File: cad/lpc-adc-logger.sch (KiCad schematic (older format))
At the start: 26 parts, among them J1 SD_CARD, J2 UART, J3 I2C, J4 ANALOG IN, J5 SWD, J6 GPIO, SW2 RESET, SW3 FLUSH, U1 LPC1114FN28

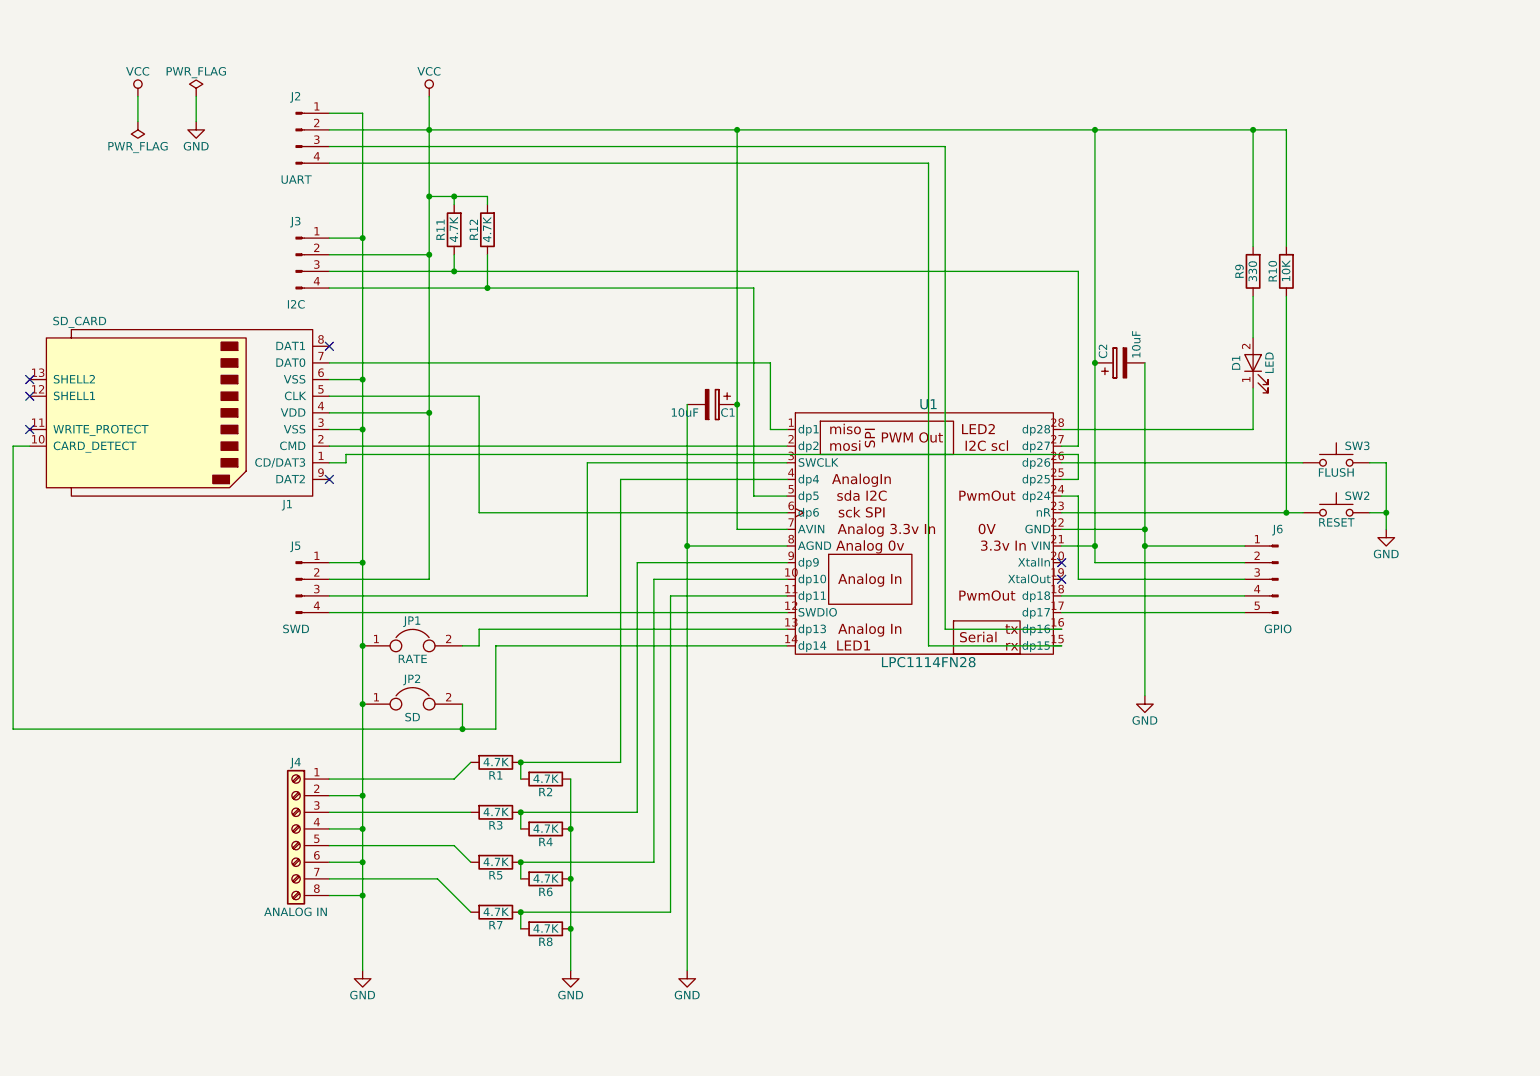
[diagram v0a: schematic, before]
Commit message: [WIP] Added SPI header.
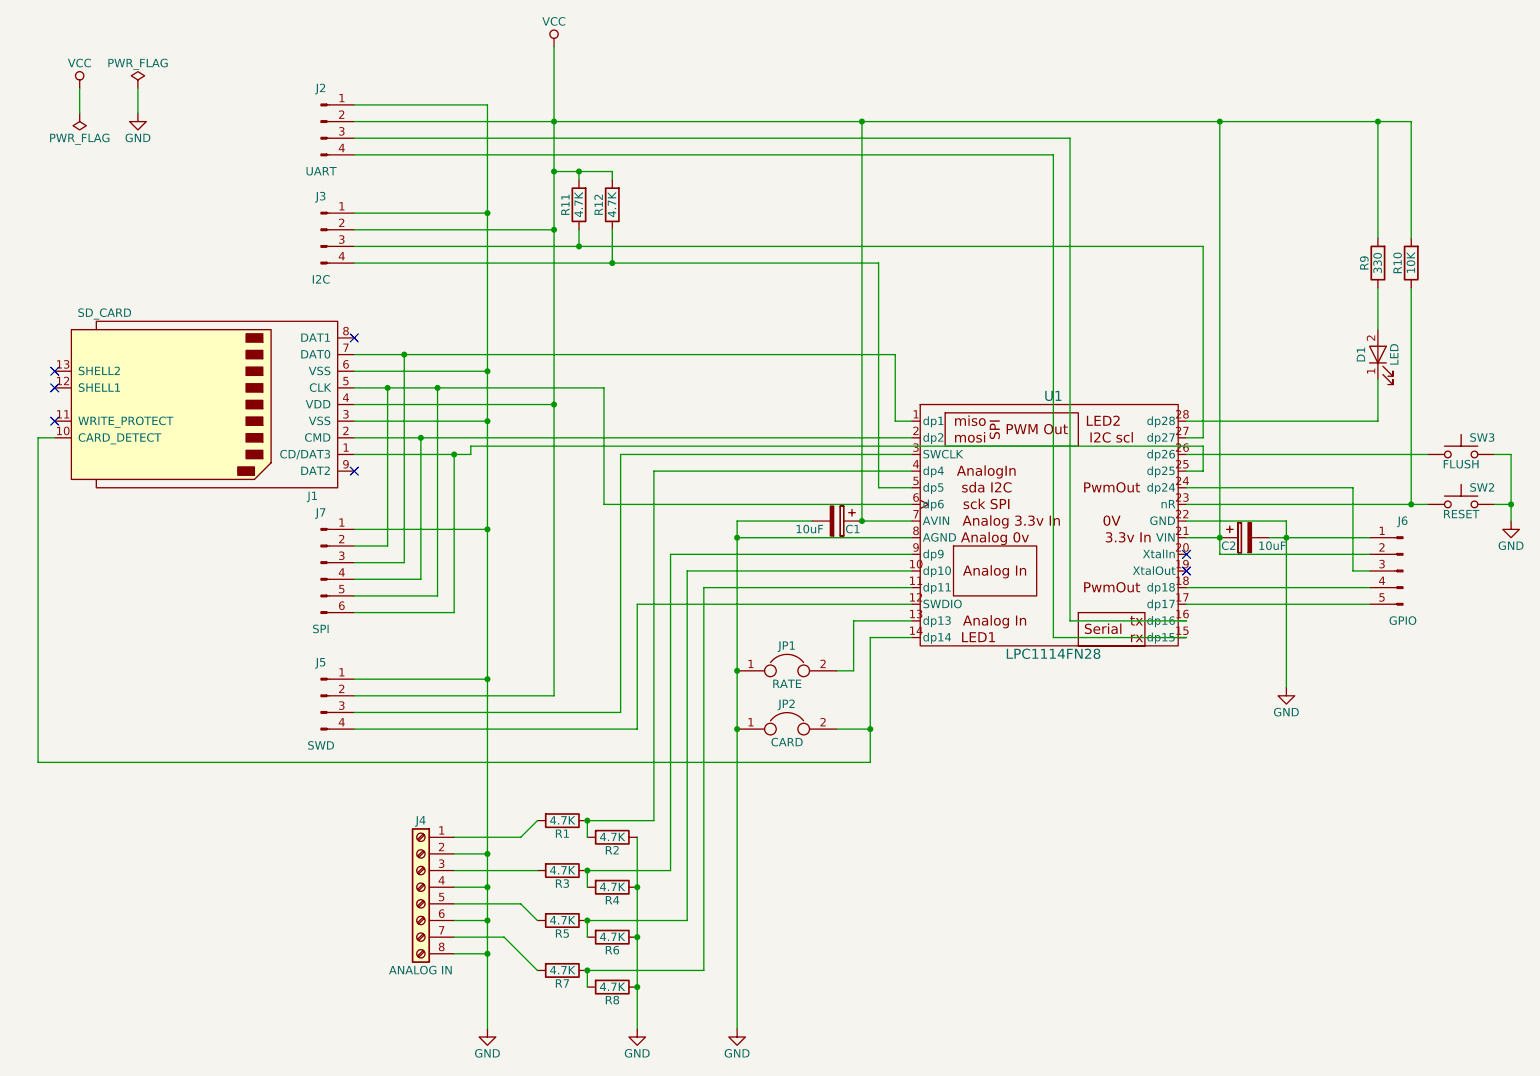
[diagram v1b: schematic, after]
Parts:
- added J7: SPI, Pin_Headers:Pin_Header_Straight_1x06_Pitch2.54mm, symbol Conn_01x06_Male
- JP2: value SD -> CARD
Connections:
- net GND: now also J7.1 (Pin_1)
- net at J1.7 (DAT0), U1.1 (dp1): now also J7.3 (Pin_3)
- net at J1.2 (CMD), U1.2 (dp2): now also J7.4 (Pin_4)
- net at J1.1 (CD/DAT3), U1.25 (dp25): now also J7.6 (Pin_6)
- net at J1.5 (CLK), U1.6 (dp6): now also J7.2 (Pin_2), J7.5 (Pin_5)
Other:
- moved on the sheet: C1, C2, D1, J1, J2, J3, J4, J5, J6, JP1, JP2, R1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
